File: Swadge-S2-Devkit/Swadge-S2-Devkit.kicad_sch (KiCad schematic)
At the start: 91 parts, among them J1 LED, J2 DEBUG, P1 USB_C_Plug_USB2.0, Q1 PMOS, SW1 TS-1109S-A-A, SW2 TS-1109S-A-A, SW3 TS-1109S-A-A, SW4 TS-1109S-A-A, SW5 TS-1109S-A-A, SW6 TS-1109S-A-A, SW7 B3FS-4002P, SW8 B3FS-4002P, SW9 SW_SPDT_1825232-1, U1 ESP32-S2-SOLO, U10 GENERIC_LDO_2.8, U11 art_melee_logo, U12 art_select_start, U13 art_squarewavebird, U14 RB017A1505A_Connector, U15 RB0154A1201A, U16 Controller_Shields, U2 RB017A1505A, U3 MT3410, U5 art_xy_buttons, U6 art_20th_logo, U7 art_d_pad, U8 art_eyebrow

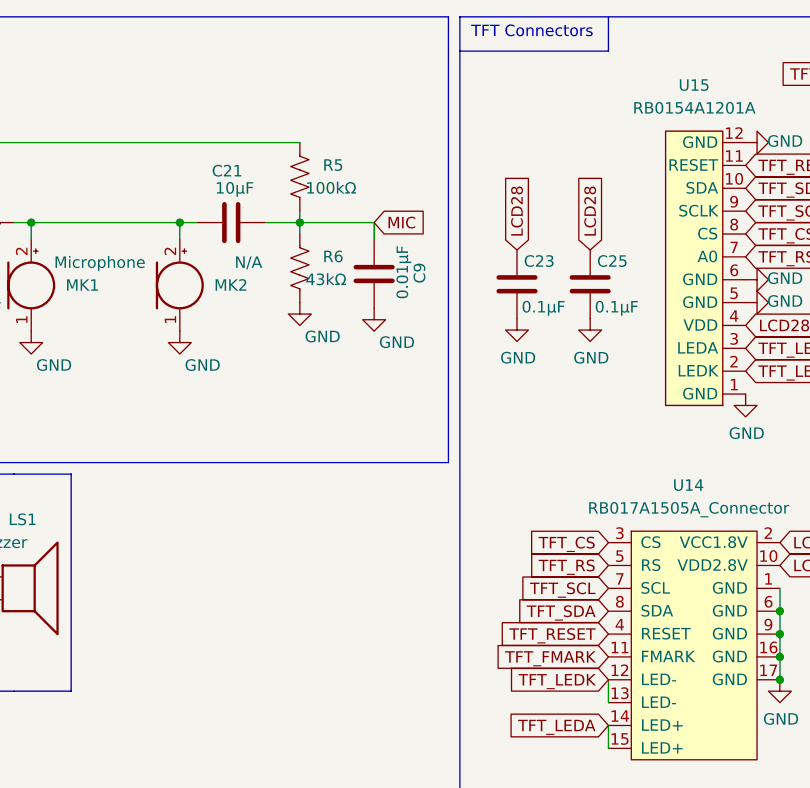
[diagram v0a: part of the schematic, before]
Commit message: update design
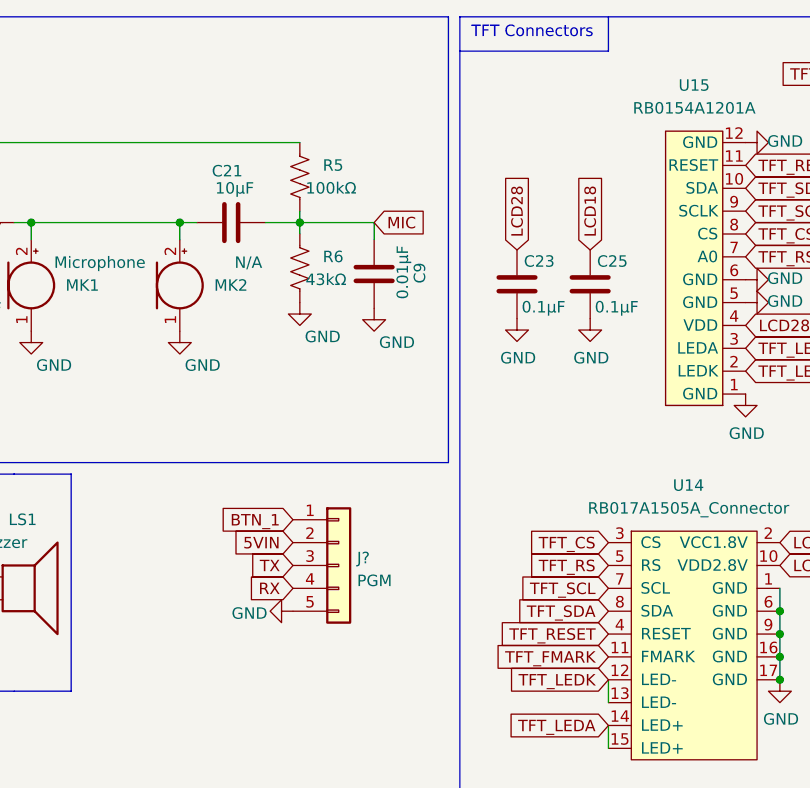
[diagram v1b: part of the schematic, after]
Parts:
- added J?: PGM, Connector_PinHeader_2.54mm:PinHeader_1x05_P2.54mm_Vertical, symbol Connector_Generic:Conn_01x05
- R8, R9: LCSC C15402 -> C21189
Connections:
- net 5VIN: now also J?.2 (Pin_2)
- net BTN_1: now also J?.1 (Pin_1)
- net GND: now also J?.5 (Pin_5)
- net LCD18: now also C25.1
- net LCD28: no longer C25.1
- net RX: now also J?.4 (Pin_4)
- net TX: now also J?.3 (Pin_3)
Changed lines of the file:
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@@
     )
   )
-  (global_label "LCD28" (shape input) (at 300.228 38.608 90) (fields_autoplaced)
-    (effects (font (size 1.27 1.27)) (justify left))
-    (property "Intersheet References" "${INTERSHEET_REFS}" (id 0) (at 300.3074 30.2078 90)
-      (effects (font (size 1.27 1.27)) (justify left) hide)
-    )
-  )
   (global_label "TOUCH_3" (shape input) (at 175.26 151.13 180) (fields_autoplaced)
     (effects (font (size 1.27 1.27)) (justify right))
@@
     )
   )
+  (global_label "5VIN" (shape input) (at 267.208 71.12 180) (fields_autoplaced)
+    (effects (font (size 1.27 1.27)) (justify right))
+    (property "Intersheet References" "${INTERSHEET_REFS}" (id 0) (at 260.5616 71.1994 0)
+      (effects (font (size 1.27 1.27)) (justify right) hide)
+    )
+  )
   (global_label "LCD28" (shape input) (at 309.372 149.86 0) (fields_autoplaced)
     (effects (font (size 1.27 1.27)) (justify left))
@@
     )
   )
+  (global_label "TX" (shape input) (at 267.208 73.66 180) (fields_autoplaced)
+    (effects (font (size 1.27 1.27)) (justify right))
+    (property "Intersheet References" "${INTERSHEET_REFS}" (id 0) (at 262.6178 73.7394 0)
+      (effects (font (size 1.27 1.27)) (justify right) hide)
+    )
+  )
   (global_label "TOUCH_1" (shape input) (at 44.45 59.69 180) (fields_autoplaced)
     (effects (font (size 1.27 1.27)) (justify right))
@@
     )
   )
+  (global_label "RX" (shape input) (at 267.208 76.2 180) (fields_autoplaced)
+    (effects (font (size 1.27 1.27)) (justify right))
+    (property "Intersheet References" "${INTERSHEET_REFS}" (id 0) (at 262.3154 76.2794 0)
+      (effects (font (size 1.27 1.27)) (justify right) hide)
+    )
+  )
   (global_label "TFT_RS" (shape input) (at 302.26 73.66 180) (fields_autoplaced)
     (effects (font (size 1.27 1.27)) (justify right))
@@
     )
   )
+  (global_label "LCD18" (shape input) (at 300.228 38.608 90) (fields_autoplaced)
+    (effects (font (size 1.27 1.27)) (justify left))
+    (property "Intersheet References" "${INTERSHEET_REFS}" (id 0) (at 300.3074 30.2078 90)
+      (effects (font (size 1.27 1.27)) (justify left) hide)
+    )
+  )
   (global_label "TFT_CS" (shape input) (at 302.26 71.12 180) (fields_autoplaced)
     (effects (font (size 1.27 1.27)) (justify right))
@@
     )
   )
+  (global_label "BTN_1" (shape input) (at 267.208 68.58 180) (fields_autoplaced)
+    (effects (font (size 1.27 1.27)) (justify right))
+    (property "Intersheet References" "${INTERSHEET_REFS}" (id 0) (at 259.0497 68.5006 0)
+      (effects (font (size 1.27 1.27)) (justify right) hide)
+    )
+  )
   (global_label "LCD18" (shape input) (at 321.31 71.12 0) (fields_autoplaced)
     (effects (font (size 1.27 1.27)) (justify left))
@@
       (effects (font (size 1.27 1.27)) hide)
     )
-    (property "LCSC" "C15402" (id 7) (at 325.12 106.426 0)
+    (property "LCSC" "C21189" (id 7) (at 325.12 106.426 0)
       (effects (font (size 1.27 1.27)) hide)
     )
@@
     (pin "1")
   )
+  (symbol (lib_id "Connector_Generic:Conn_01x05") (at 272.288 73.66 0) (unit 1)
+    (in_bom yes) (on_board yes) (fields_autoplaced)
+    (property "Reference" "J?" (id 0) (at 274.32 72.8253 0)
+      (effects (font (size 1.27 1.27)) (justify left))
+    )
+    (property "Value" "PGM" (id 1) (at 274.32 75.3622 0)
+      (effects (font (size 1.27 1.27)) (justify left))
+    )
+    (property "Footprint" "Connector_PinHeader_2.54mm:PinHeader_1x05_P2.54mm_Vertical" (id 2) (at 272.288 73.66 0)
+      (effects (font (size 1.27 1.27)) hide)
+    )
+    (property "Datasheet" "~" (id 3) (at 272.288 73.66 0)
+      (effects (font (size 1.27 1.27)) hide)
+    )
+    (property "LCSC" "NP" (id 4) (at 272.288 73.66 0)
+      (effects (font (size 1.27 1.27)) hide)
+    )
+    (pin "1")
+    (pin "2")
+    (pin "3")
+    (pin "4")
+    (pin "5")
+  )
   (symbol (lib_id "Swadge_Parts:Microphone") (at 238.125 42.545 0) (unit 1)
     (in_bom yes) (on_board yes)
@@
     (pin "1")
   )
+  (symbol (lib_id "Swadge_Parts:GND") (at 267.208 78.74 270) (unit 1)
+    (in_bom yes) (on_board yes)
+    (property "Reference" "#PWR?" (id 0) (at 260.858 78.74 0)
+      (effects (font (size 1.27 1.27)) hide)
+    )
+    (property "Value" "GND" (id 1) (at 262.382 78.994 90))
+    (property "Footprint" "" (id 2) (at 267.208 78.74 0)
+      (effects (font (size 1.27 1.27)) hide)
+    )
+    (property "Datasheet" "" (id 3) (at 267.208 78.74 0)
+      (effects (font (size 1.27 1.27)) hide)
+    )
+    (pin "1")
+  )
   (symbol (lib_name "SK6812SIDE_2") (lib_id "Swadge_Parts:SK6812SIDE") (at 41.91 138.43 0) (unit 1)
     (in_bom yes) (on_board yes)
@@
       (effects (font (size 1.27 1.27)) hide)
     )
-    (property "LCSC" "C15402" (id 7) (at 323.85 139.7 0)
+    (property "LCSC" "C21189" (id 7) (at 323.85 139.7 0)
       (effects (font (size 1.27 1.27)) hide)
     )
@@
       (reference "#PWR0116") (unit 1) (value "GND") (footprint "")
     )
+    (path "/b0c4b47b-f7ae-4d66-b619-e92865675556"
+      (reference "#PWR?") (unit 1) (value "GND") (footprint "")
+    )
     (path "/6efbac4e-4c48-4d85-b138-3166666d2e76"
       (reference "BT1") (unit 1) (value "Battery") (footprint "Swadge_Parts:2460")
@@
       (reference "J2") (unit 1) (value "DEBUG") (footprint "Connector_PinHeader_2.54mm:PinHeader_2x10_P2.54mm_Vertical")
     )
+    (path "/a55c1b99-3293-490d-831c-cf15a08bdfa8"
+      (reference "J?") (unit 1) (value "PGM") (footprint "Connector_PinHeader_2.54mm:PinHeader_1x05_P2.54mm_Vertical")
+    )
     (path "/3e011cdb-c151-46b2-9f97-ba78518661fd"
